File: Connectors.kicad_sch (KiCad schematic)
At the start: 14 parts, among them J1 A, J10 4900, J11 4900, J12 4900, J13 4900, J14 4900, J2 B, J3 C, J4 Conn_02x07_Odd_Even, J5 4900, J6 4900, J7 4900, J8 Conn_02x02_Odd_Even, J9 4900

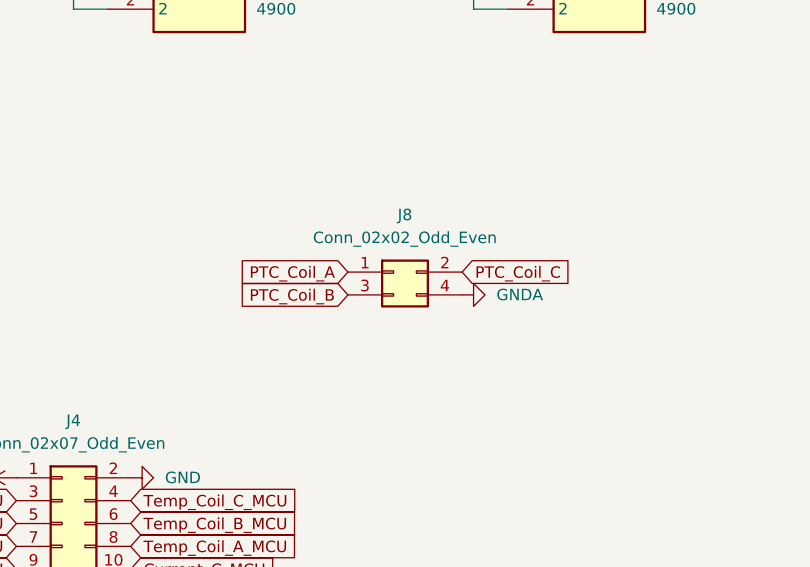
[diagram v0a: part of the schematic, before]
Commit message: Собираю документацию
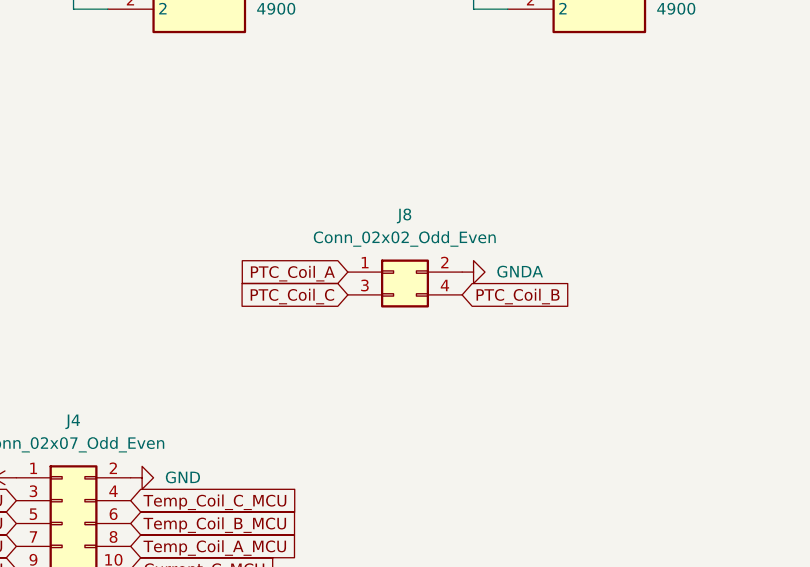
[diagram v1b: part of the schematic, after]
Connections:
- net GNDA: now also J8.2 (Pin_2); no longer J8.4 (Pin_4)
- net PTC_Coil_B: now also J8.4 (Pin_4); no longer J8.3 (Pin_3)
- net PTC_Coil_C: now also J8.3 (Pin_3); no longer J8.2 (Pin_2)
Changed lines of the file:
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@@
     )
   )
-  (global_label "PTC_Coil_C" (shape input) (at 186.69 95.25 0) (fields_autoplaced)
-    (effects (font (size 1.27 1.27)) (justify left))
-    (property "Intersheetrefs" "${INTERSHEET_REFS}" (at 200.077 95.25 0)
-      (effects (font (size 1.27 1.27)) (justify left) hide)
+  (global_label "PTC_Coil_C" (shape input) (at 173.99 97.79 180) (fields_autoplaced)
+    (effects (font (size 1.27 1.27)) (justify right))
+    (property "Intersheetrefs" "${INTERSHEET_REFS}" (at 160.603 97.79 0)
+      (effects (font (size 1.27 1.27)) (justify right) hide)
     )
   )
@@
     )
   )
-  (global_label "PTC_Coil_B" (shape input) (at 173.99 97.79 180) (fields_autoplaced)
-    (effects (font (size 1.27 1.27)) (justify right))
-    (property "Intersheetrefs" "${INTERSHEET_REFS}" (at 160.603 97.79 0)
-      (effects (font (size 1.27 1.27)) (justify right) hide)
+  (global_label "PTC_Coil_B" (shape input) (at 186.69 97.79 0) (fields_autoplaced)
+    (effects (font (size 1.27 1.27)) (justify left))
+    (property "Intersheetrefs" "${INTERSHEET_REFS}" (at 200.077 97.79 0)
+      (effects (font (size 1.27 1.27)) (justify left) hide)
     )
   )
@@
     )
   )
-  (symbol (lib_id "power:GNDA") (at 186.69 97.79 90) (unit 1)
-    (in_bom yes) (on_board yes) (dnp no) (fields_autoplaced)
-    (property "Reference" "#PWR038" (at 193.04 97.79 0)
-      (effects (font (size 1.27 1.27)) hide)
-    )
-    (property "Value" "GNDA" (at 190.5 97.79 90)
+  (symbol (lib_id "power:GNDA") (at 186.69 95.25 90) (unit 1)
+    (in_bom yes) (on_board yes) (dnp no) (fields_autoplaced)
+    (property "Reference" "#PWR038" (at 193.04 95.25 0)
+      (effects (font (size 1.27 1.27)) hide)
+    )
+    (property "Value" "GNDA" (at 190.5 95.25 90)
       (effects (font (size 1.27 1.27)) (justify right))
     )
-    (property "Footprint" "" (at 186.69 97.79 0)
-      (effects (font (size 1.27 1.27)) hide)
-    )
-    (property "Datasheet" "" (at 186.69 97.79 0)
-      (effects (font (size 1.27 1.27)) hide)
-    )
+    (property "Footprint" "" (at 186.69 95.25 0)
+      (effects (font (size 1.27 1.27)) hide)
+    )
+    (property "Datasheet" "" (at 186.69 95.25 0)
+      (effects (font (size 1.27 1.27)) hide)
+    )

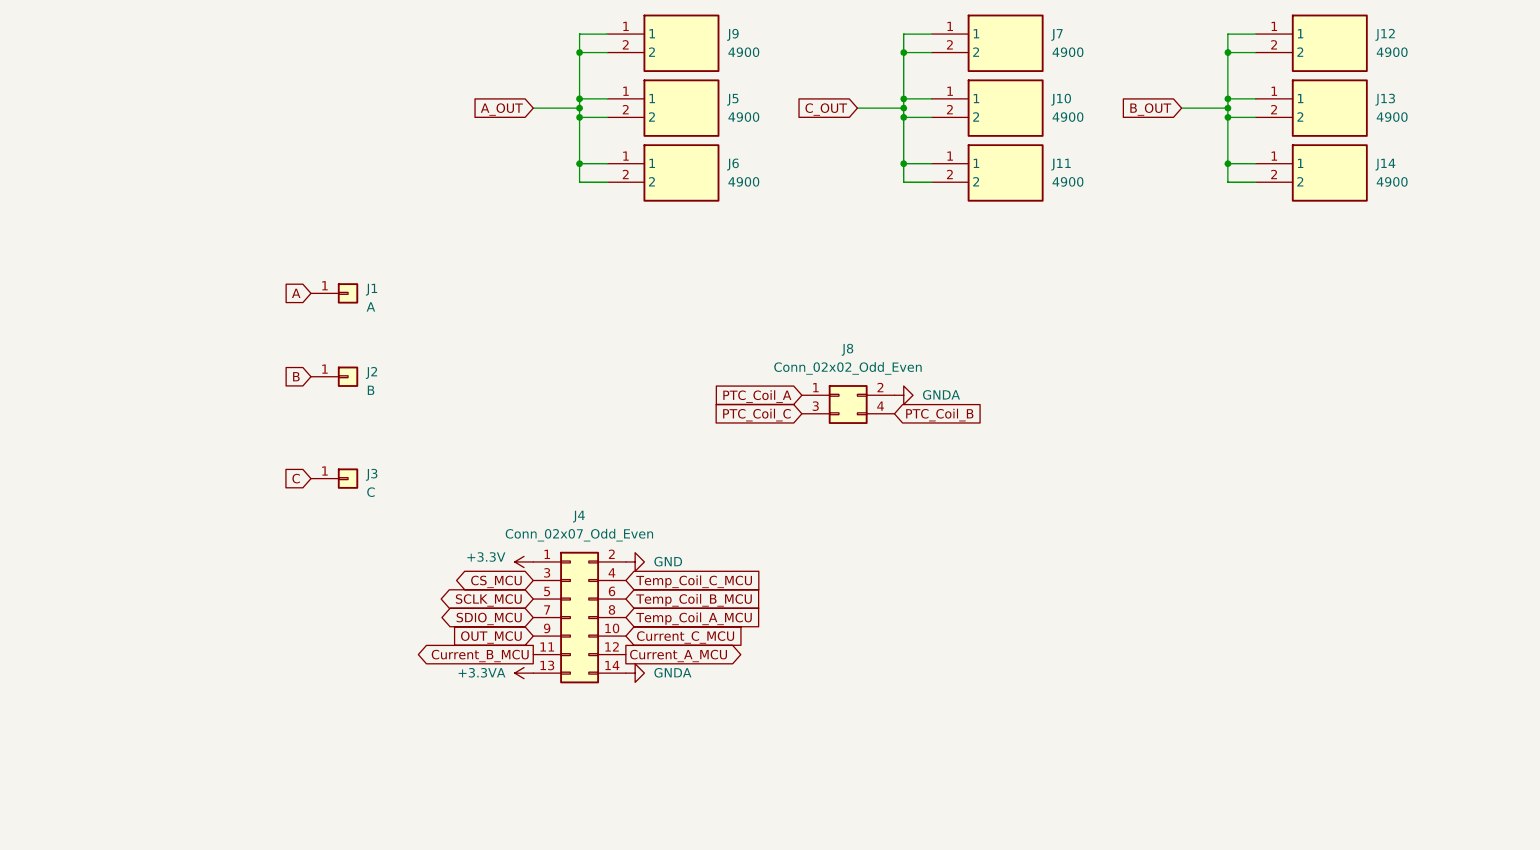
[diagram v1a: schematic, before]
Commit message: ...
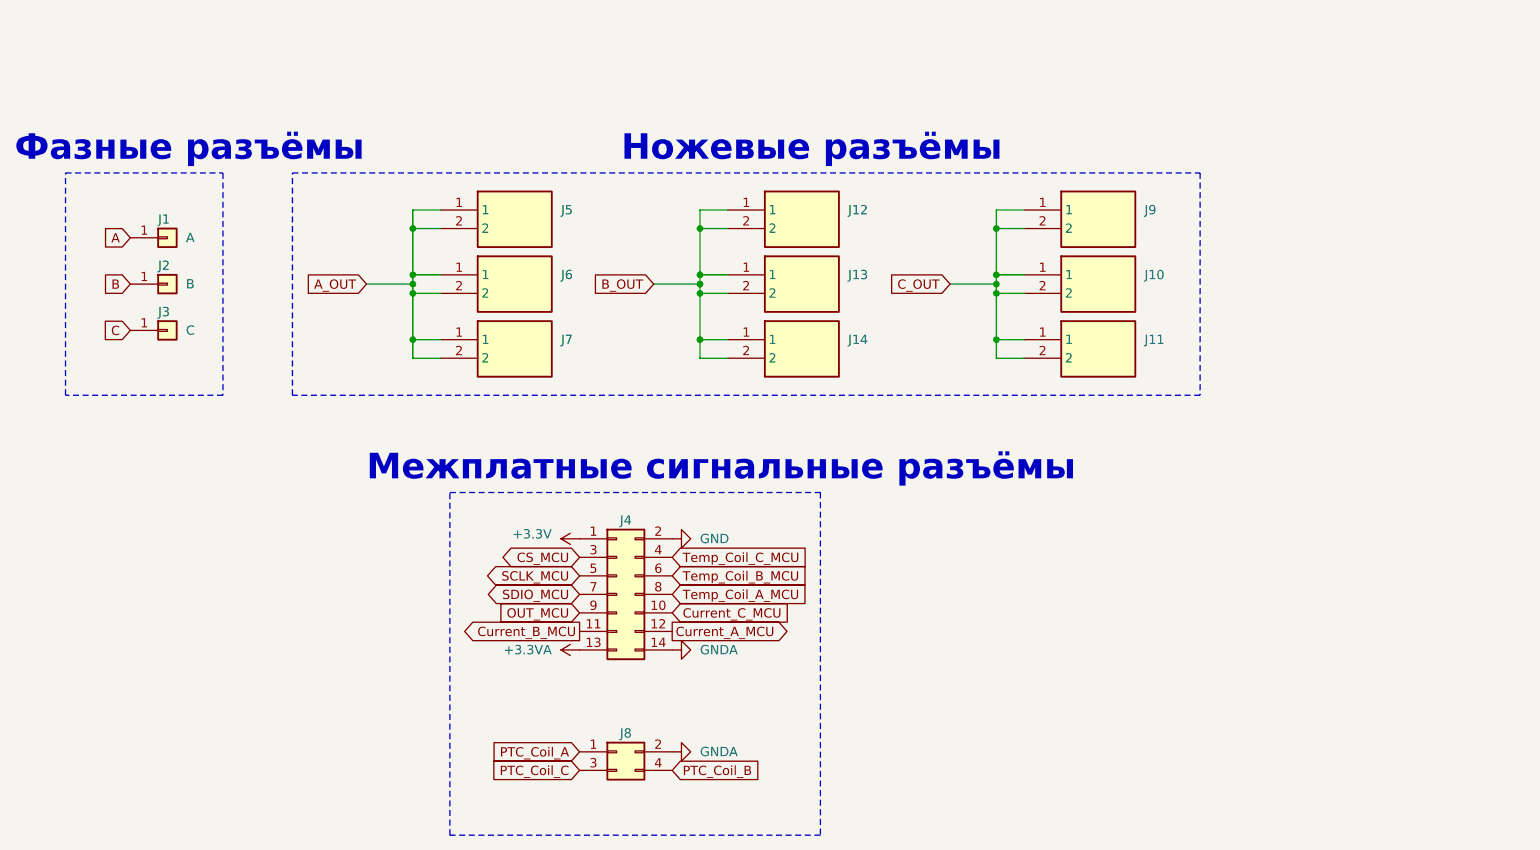
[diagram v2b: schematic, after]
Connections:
- net A_OUT: now also J7.1, J7.2; no longer J9.1, J9.2
- net C_OUT: now also J9.1, J9.2; no longer J7.1, J7.2
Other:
- note added: "Межплатные сигнальные разъёмы"
- note added: "Ножевые разъёмы"
- note added: "Фазные разъёмы"

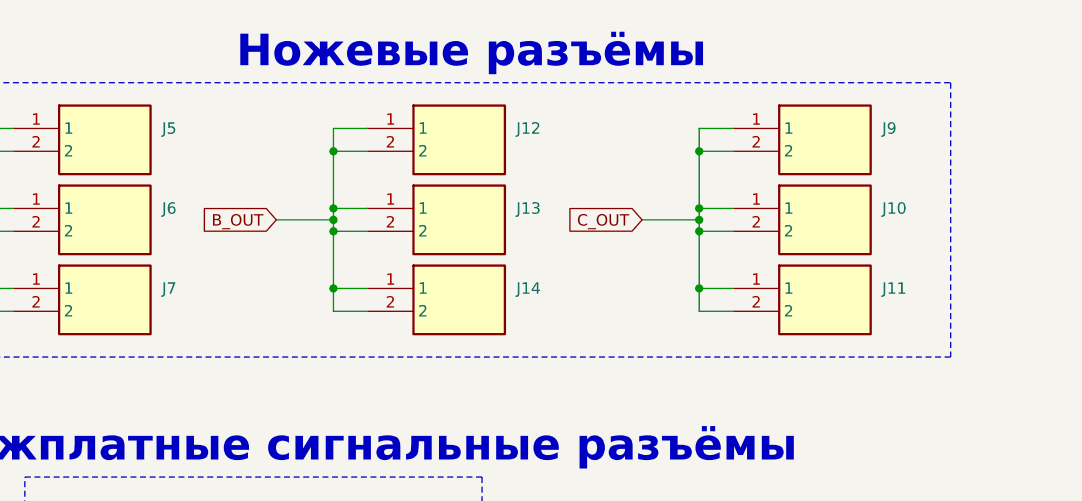
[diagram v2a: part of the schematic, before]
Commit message: Версия под отчёт
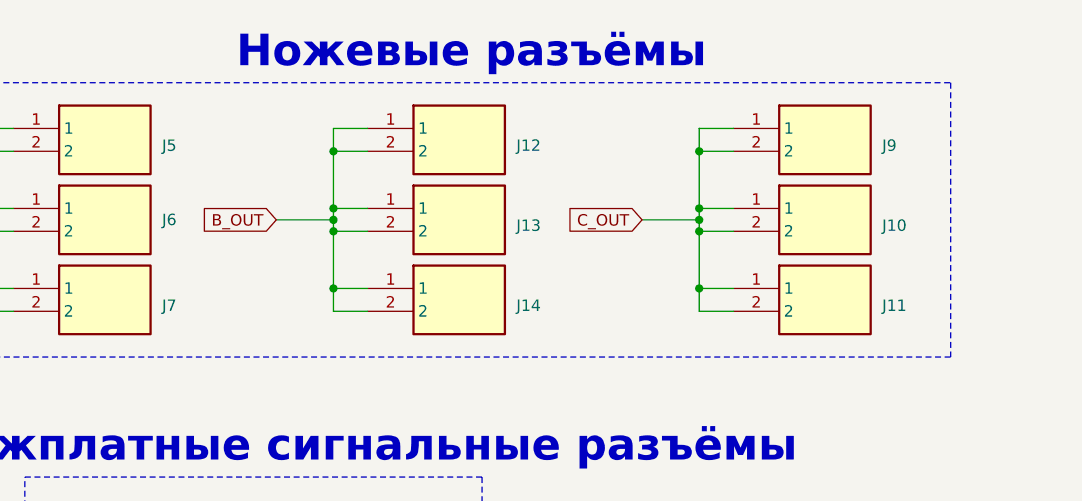
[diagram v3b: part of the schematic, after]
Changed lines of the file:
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@@
         )
         (path "/69677e3f-3942-4c93-9a5c-92669e2df5eb/555e8538-1d60-4a85-8162-4c8254aec889"
-          (reference "J11") (unit 1)
+          (reference "J3") (unit 1)
         )
         (path "/69677e3f-3942-4c93-9a5c-92669e2df5eb/25ee8137-5200-4a92-a72b-f10625be9855"
@@
   (symbol (lib_id "4900:4900") (at 163.83 69.85 0) (unit 1)
     (in_bom yes) (on_board yes) (dnp no) (fields_autoplaced)
-    (property "Reference" "J12" (at 180.34 69.85 0)
+    (property "Reference" "J12" (at 180.34 71.7549 0)
       (effects (font (size 1.27 1.27)) (justify left))
     )
@@
         )
         (path "/69677e3f-3942-4c93-9a5c-92669e2df5eb/555e8538-1d60-4a85-8162-4c8254aec889"
-          (reference "J2") (unit 1)
+          (reference "J12") (unit 1)
         )
         (path "/69677e3f-3942-4c93-9a5c-92669e2df5eb/25ee8137-5200-4a92-a72b-f10625be9855"
@@
   (symbol (lib_id "4900:4900") (at 204.47 87.63 0) (unit 1)
     (in_bom yes) (on_board yes) (dnp no) (fields_autoplaced)
-    (property "Reference" "J11" (at 220.98 87.63 0)
+    (property "Reference" "J11" (at 220.98 89.5349 0)
       (effects (font (size 1.27 1.27)) (justify left))
     )
@@
         )
         (path "/69677e3f-3942-4c93-9a5c-92669e2df5eb/555e8538-1d60-4a85-8162-4c8254aec889"
-          (reference "J14") (unit 1)
+          (reference "J11") (unit 1)
         )
         (path "/69677e3f-3942-4c93-9a5c-92669e2df5eb/25ee8137-5200-4a92-a72b-f10625be9855"
@@
   )
   (symbol (lib_id "4900:4900") (at 124.46 78.74 0) (unit 1)
-    (in_bom yes) (on_board yes) (dnp no) (fields_autoplaced)
-    (property "Reference" "J6" (at 140.97 78.74 0)
+    (in_bom yes) (on_board yes) (dnp no)
+    (property "Reference" "J6" (at 140.97 80.01 0)
       (effects (font (size 1.27 1.27)) (justify left))
     )
@@
         )
         (path "/69677e3f-3942-4c93-9a5c-92669e2df5eb/555e8538-1d60-4a85-8162-4c8254aec889"
-          (reference "J10") (unit 1)
+          (reference "J2") (unit 1)
         )
         (path "/69677e3f-3942-4c93-9a5c-92669e2df5eb/25ee8137-5200-4a92-a72b-f10625be9855"
@@
   (symbol (lib_id "4900:4900") (at 163.83 87.63 0) (unit 1)
     (in_bom yes) (on_board yes) (dnp no) (fields_autoplaced)
-    (property "Reference" "J14" (at 180.34 87.63 0)
+    (property "Reference" "J14" (at 180.34 89.5349 0)
       (effects (font (size 1.27 1.27)) (justify left))
     )
@@
         )
         (path "/69677e3f-3942-4c93-9a5c-92669e2df5eb/555e8538-1d60-4a85-8162-4c8254aec889"
-          (reference "J13") (unit 1)
+          (reference "J14") (unit 1)
         )
         (path "/69677e3f-3942-4c93-9a5c-92669e2df5eb/25ee8137-5200-4a92-a72b-f10625be9855"
@@
   (symbol (lib_id "4900:4900") (at 124.46 69.85 0) (unit 1)
     (in_bom yes) (on_board yes) (dnp no) (fields_autoplaced)
-    (property "Reference" "J5" (at 140.97 69.85 0)
+    (property "Reference" "J5" (at 140.97 71.7549 0)
       (effects (font (size 1.27 1.27)) (justify left))
     )
@@
         )
         (path "/69677e3f-3942-4c93-9a5c-92669e2df5eb/555e8538-1d60-4a85-8162-4c8254aec889"
-          (reference "J1") (unit 1)
+          (reference "J5") (unit 1)
         )
         (path "/69677e3f-3942-4c93-9a5c-92669e2df5eb/25ee8137-5200-4a92-a72b-f10625be9855"
@@
   (symbol (lib_id "4900:4900") (at 204.47 69.85 0) (unit 1)
     (in_bom yes) (on_board yes) (dnp no) (fields_autoplaced)
-    (property "Reference" "J9" (at 220.98 69.85 0)
+    (property "Reference" "J9" (at 220.98 71.7549 0)
       (effects (font (size 1.27 1.27)) (justify left))
     )
@@
         )
         (path "/69677e3f-3942-4c93-9a5c-92669e2df5eb/555e8538-1d60-4a85-8162-4c8254aec889"
-          (reference "J3") (unit 1)
+          (reference "J7") (unit 1)
         )
         (path "/69677e3f-3942-4c93-9a5c-92669e2df5eb/25ee8137-5200-4a92-a72b-f10625be9855"
@@
   (symbol (lib_id "4900:4900") (at 163.83 78.74 0) (unit 1)
     (in_bom yes) (on_board yes) (dnp no) (fields_autoplaced)
-    (property "Reference" "J13" (at 180.34 78.74 0)
+    (property "Reference" "J13" (at 180.34 80.6449 0)
       (effects (font (size 1.27 1.27)) (justify left))
     )
@@
         )
         (path "/69677e3f-3942-4c93-9a5c-92669e2df5eb/555e8538-1d60-4a85-8162-4c8254aec889"
+          (reference "J13") (unit 1)
+        )
+        (path "/69677e3f-3942-4c93-9a5c-92669e2df5eb/25ee8137-5200-4a92-a72b-f10625be9855"
+          (reference "J20") (unit 1)
+        )
+      )
+    )
+  )
+  (symbol (lib_id "4900:4900") (at 124.46 87.63 0) (unit 1)
+    (in_bom yes) (on_board yes) (dnp no) (fields_autoplaced)
+    (property "Reference" "J7" (at 140.97 89.5349 0)
+      (effects (font (size 1.27 1.27)) (justify left))
+    )
+    (property "Value" "4900" (at 140.97 90.17 0)
+      (effects (font (size 1.27 1.27)) (justify left) hide)
+    )
+    (property "Footprint" "Connector_My:4900" (at 140.97 182.55 0)
+      (effects (font (size 1.27 1.27)) (justify left top) hide)
+    )
+    (property "Datasheet" "https://www.keyelco.com/product-pdf.cfm?p=597" (at 140.97 282.55 0)
+      (effects (font (size 1.27 1.27)) (justify left top) hide)
+    )
+    (property "Height" "10.72" (at 140.97 482.55 0)
+      (effects (font (size 1.27 1.27)) (justify left top) hide)
+    )
+    (property "Manufacturer_Name" "Keystone Electronics" (at 140.97 582.55 0)
+      (effects (font (size 1.27 1.27)) (justify left top) hide)
+    )
+    (property "Manufacturer_Part_Number" "4900" (at 140.97 682.55 0)
+      (effects (font (size 1.27 1.27)) (justify left top) hide)
+    )
+    (property "Mouser Part Number" "534-4900" (at 140.97 782.55 0)
+      (effects (font (size 1.27 1.27)) (justify left top) hide)
+    )
+    (property "Mouser Price/Stock" "https://www.mouser.co.uk/ProductDetail/Keystone-Electronics/4900?qs=lQmX4aIt5iDWRkxqjAIN4A%3D%3D" (at 140.97 882.55 0)
+      (effects (font (size 1.27 1.27)) (justify left top) hide)
+    )
+    (property "Arrow Part Number" "" (at 140.97 982.55 0)
+      (effects (font (size 1.27 1.27)) (justify left top) hide)
+    )
+    (property "Arrow Price/Stock" "" (at 140.97 1082.55 0)
+      (effects (font (size 1.27 1.27)) (justify left top) hide)
+    )
+    (pin "1")
+    (pin "2")
+    (instances
+      (project "Плата датчиков"
+        (path "/69677e3f-3942-4c93-9a5c-92669e2df5eb"
           (reference "J7") (unit 1)
         )
-        (path "/69677e3f-3942-4c93-9a5c-92669e2df5eb/25ee8137-5200-4a92-a72b-f10625be9855"
-          (reference "J20") (unit 1)
-        )
-      )
-    )
-  )
-  (symbol (lib_id "4900:4900") (at 124.46 87.63 0) (unit 1)
-    (in_bom yes) (on_board yes) (dnp no) (fields_autoplaced)
-    (property "Reference" "J7" (at 140.97 87.63 0)
-      (effects (font (size 1.27 1.27)) (justify left))
-    )
-    (property "Value" "4900" (at 140.97 90.17 0)
-      (effects (font (size 1.27 1.27)) (justify left) hide)
-    )
-    (property "Footprint" "Connector_My:4900" (at 140.97 182.55 0)
-      (effects (font (size 1.27 1.27)) (justify left top) hide)
-    )
-    (property "Datasheet" "https://www.keyelco.com/product-pdf.cfm?p=597" (at 140.97 282.55 0)
-      (effects (font (size 1.27 1.27)) (justify left top) hide)
-    )
-    (property "Height" "10.72" (at 140.97 482.55 0)
-      (effects (font (size 1.27 1.27)) (justify left top) hide)
-    )
-    (property "Manufacturer_Name" "Keystone Electronics" (at 140.97 582.55 0)
-      (effects (font (size 1.27 1.27)) (justify left top) hide)
-    )
-    (property "Manufacturer_Part_Number" "4900" (at 140.97 682.55 0)
-      (effects (font (size 1.27 1.27)) (justify left top) hide)
-    )
-    (property "Mouser Part Number" "534-4900" (at 140.97 782.55 0)
-      (effects (font (size 1.27 1.27)) (justify left top) hide)
-    )
-    (property "Mouser Price/Stock" "https://www.mouser.co.uk/ProductDetail/Keystone-Electronics/4900?qs=lQmX4aIt5iDWRkxqjAIN4A%3D%3D" (at 140.97 882.55 0)
-      (effects (font (size 1.27 1.27)) (justify left top) hide)
-    )
-    (property "Arrow Part Number" "" (at 140.97 982.55 0)
-      (effects (font (size 1.27 1.27)) (justify left top) hide)
-    )
-    (property "Arrow Price/Stock" "" (at 140.97 1082.55 0)
-      (effects (font (size 1.27 1.27)) (justify left top) hide)
-    )
-    (pin "1")
-    (pin "2")
-    (instances
-      (project "Плата датчиков"
-        (path "/69677e3f-3942-4c93-9a5c-92669e2df5eb"
-          (reference "J7") (unit 1)
-        )
-        (path "/69677e3f-3942-4c93-9a5c-92669e2df5eb/555e8538-1d60-4a85-8162-4c8254aec889"
-          (reference "J12") (unit 1)
+        (path "/69677e3f-3942-4c93-9a5c-92669e2df5eb/555e8538-1d60-4a85-8162-4c8254aec889"
+          (reference "J9") (unit 1)
         )
         (path "/69677e3f-3942-4c93-9a5c-92669e2df5eb/25ee8137-5200-4a92-a72b-f10625be9855"
@@
   (symbol (lib_id "4900:4900") (at 204.47 78.74 0) (unit 1)
     (in_bom yes) (on_board yes) (dnp no) (fields_autoplaced)
-    (property "Reference" "J10" (at 220.98 78.74 0)
+    (property "Reference" "J10" (at 220.98 80.6449 0)
       (effects (font (size 1.27 1.27)) (justify left))
     )
@@
         )
         (path "/69677e3f-3942-4c93-9a5c-92669e2df5eb/555e8538-1d60-4a85-8162-4c8254aec889"
-          (reference "J9") (unit 1)
+          (reference "J10") (unit 1)
         )
         (path "/69677e3f-3942-4c93-9a5c-92669e2df5eb/25ee8137-5200-4a92-a72b-f10625be9855"
@@
         )
         (path "/69677e3f-3942-4c93-9a5c-92669e2df5eb/555e8538-1d60-4a85-8162-4c8254aec889"
-          (reference "J5") (unit 1)
-        )
-        (path "/69677e3f-3942-4c93-9a5c-92669e2df5eb/25ee8137-5200-4a92-a72b-f10625be9855"
+          (reference "J1") (unit 1)
+        )
+        (path "/69677e3f-3942-4c93-9a5c-92669e2df5eb/25ee8137-5200-4a92-a72b-f10625be9855"
